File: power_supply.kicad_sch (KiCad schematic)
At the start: 44 parts, among them IC3 TPS2115ADRBT, J2 wireless_charging, J4 tp5100, J5 BATTERY, J8 GSB1C411111DS1HR, SW2 REG_EN, U2 TPS63000, U4 TPS63000, U5 74LVC2G74

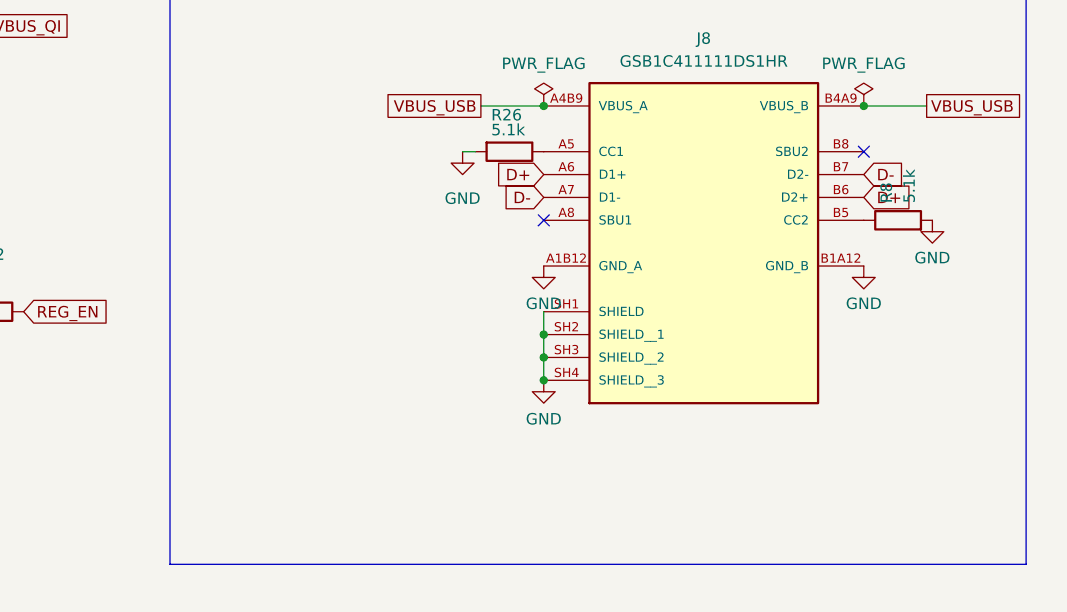
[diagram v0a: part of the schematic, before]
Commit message: -add end revision
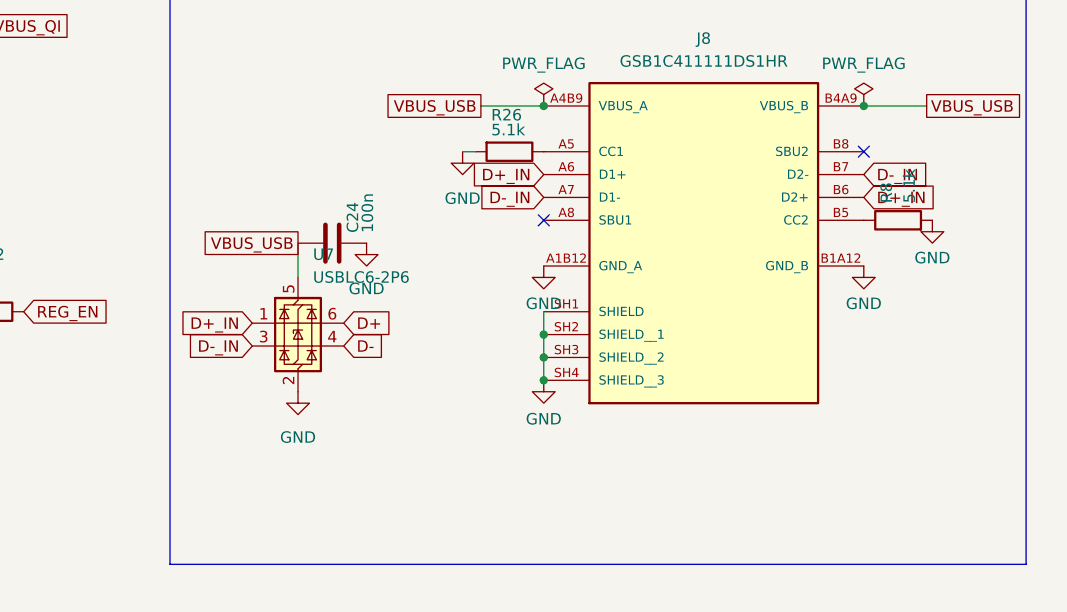
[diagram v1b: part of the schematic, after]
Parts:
- added C24: 100n, Capacitor_SMD:C_0603_1608Metric_Pad1.08x0.95mm_HandSolder, symbol Device:C
- added U7: USBLC6-2P6, Package_TO_SOT_SMD:SOT-666, symbol Power_Protection:USBLC6-2P6
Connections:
- net D+: now also U7.6 (I/O1); no longer J8.A6 (D1+), J8.B6 (D2+)
- net D-: now also U7.4 (I/O2); no longer J8.A7 (D1-), J8.B7 (D2-)
- net GND: now also C24.2, U7.2 (GND)
- net VBUS_USB: now also C24.1, U7.5 (VBUS)
- new net D+_IN: J8.A6 (D1+), J8.B6 (D2+), U7.1 (I/O1)
- new net D-_IN: J8.A7 (D1-), J8.B7 (D2-), U7.3 (I/O2)
